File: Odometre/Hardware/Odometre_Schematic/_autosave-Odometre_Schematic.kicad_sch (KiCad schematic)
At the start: 9 parts, among them IC1 STM32C092FCP6, J1 Conn_01x04_Pin, J2 Conn_01x08_Pin, U1 MCP2562-E-SN, U2 LM1117DT-3.3

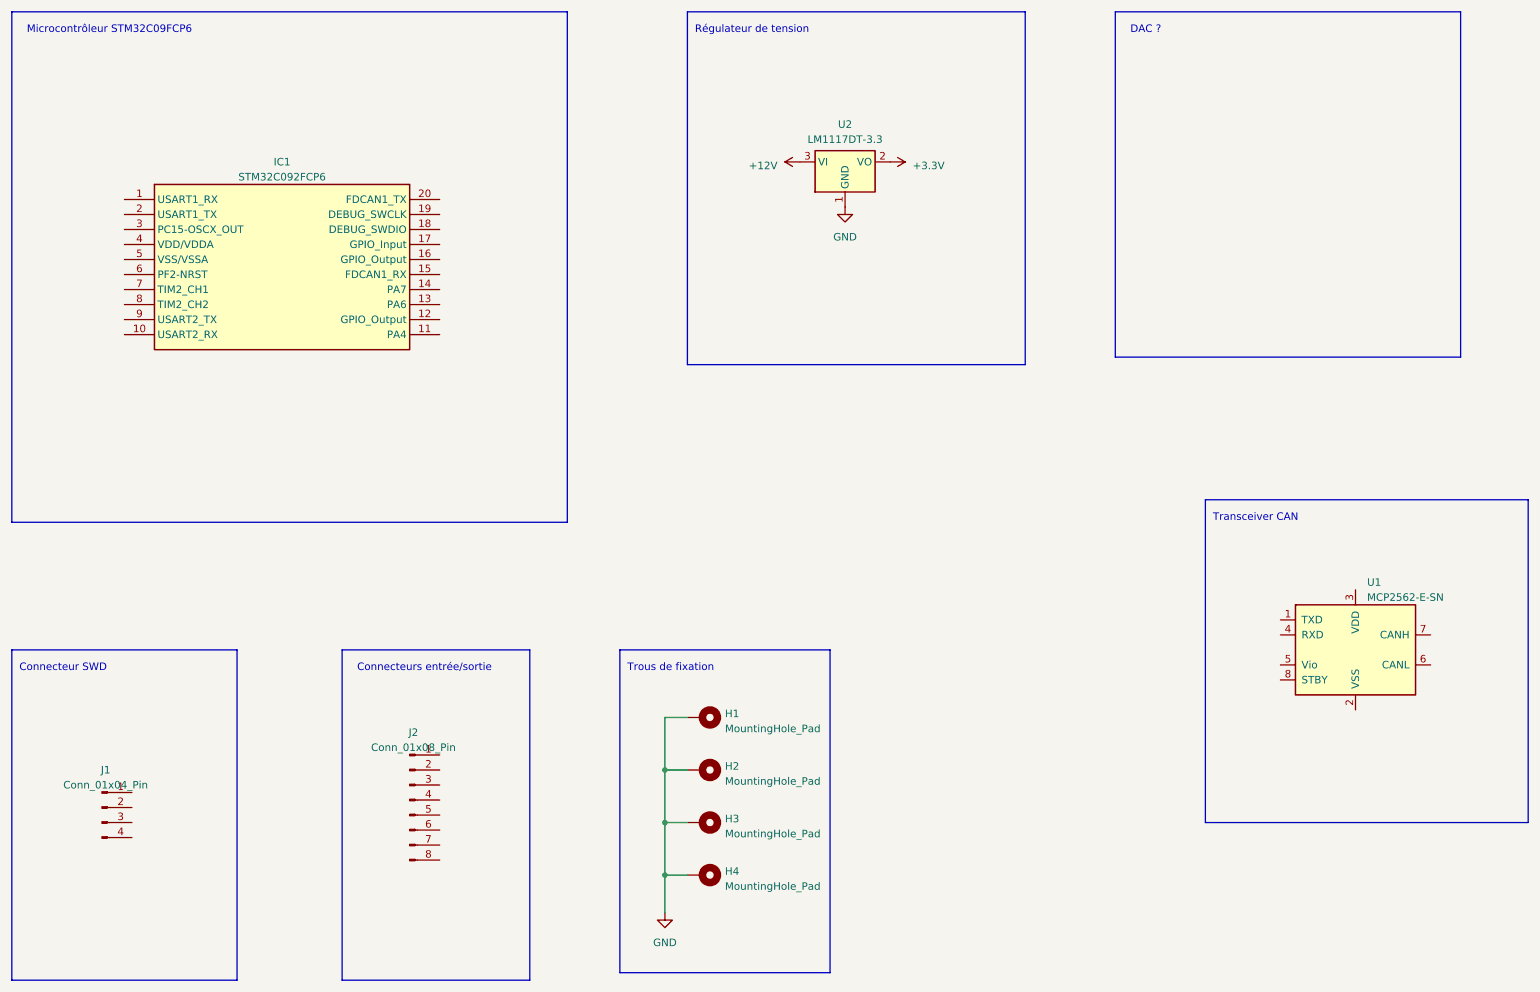
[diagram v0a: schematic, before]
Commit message: autosave kicad
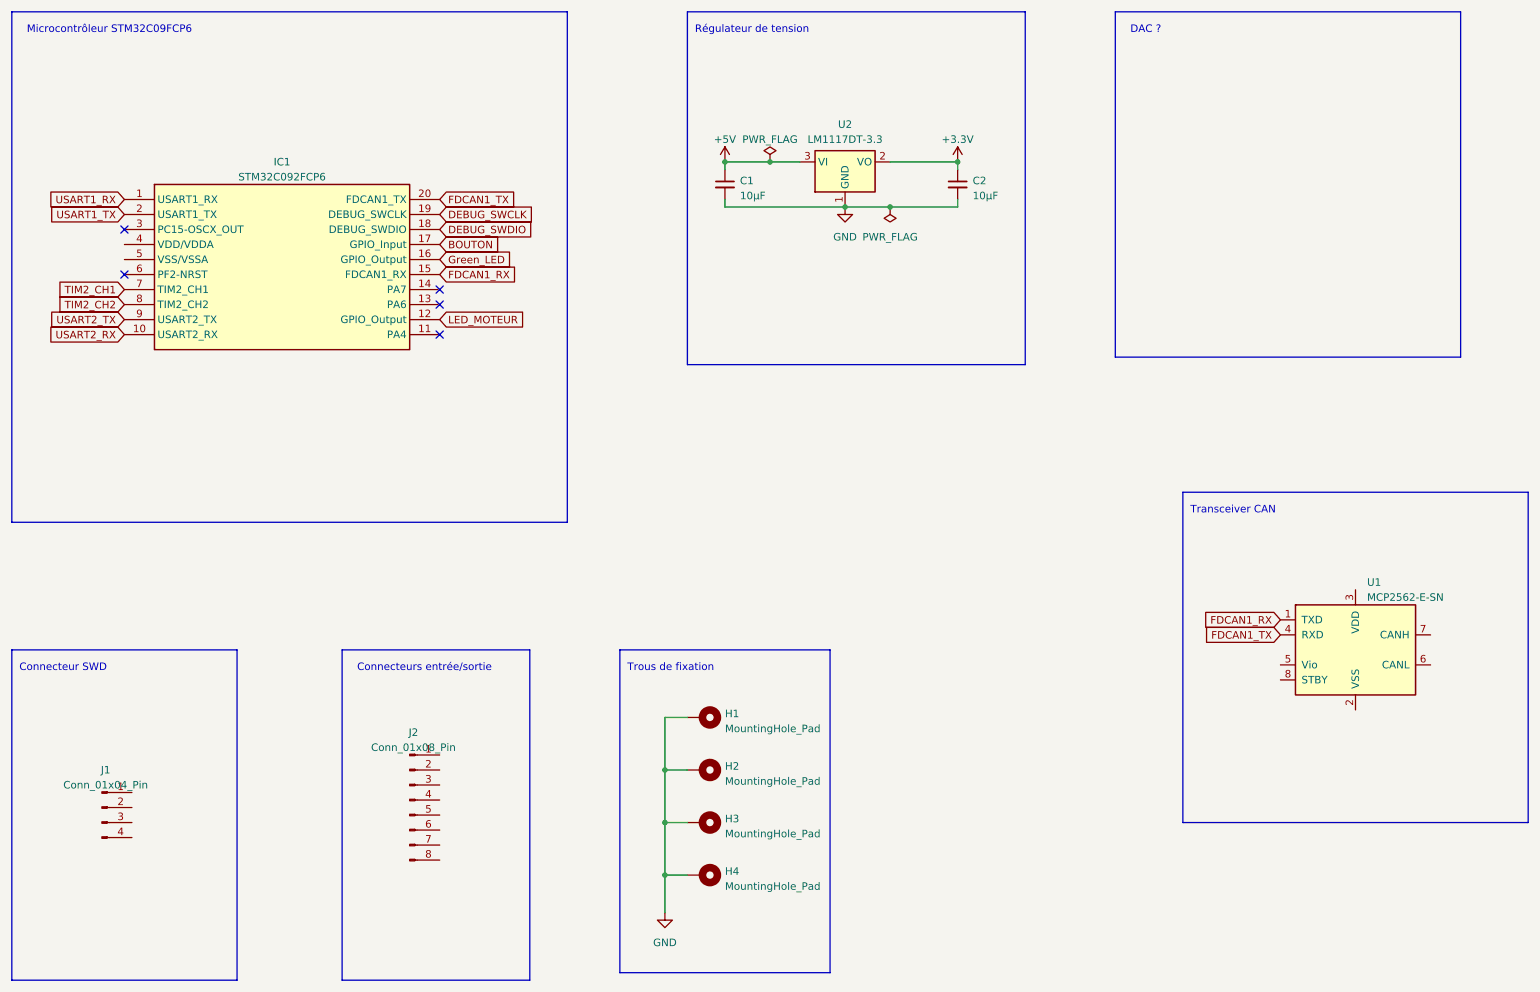
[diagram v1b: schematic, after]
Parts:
- added C1, C2: 10µF, symbol Device:C_Small
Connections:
- net +3.3V: now also C2.1
- net GND: now also C1.2, C2.2
- net FDCAN1_RX: now reaches U1.1 (TXD)
- net FDCAN1_RX: now also IC1.15 (FDCAN1_RX)
- net FDCAN1_TX: now reaches U1.4 (RXD)
- net FDCAN1_TX: now also IC1.20 (FDCAN1_TX)
- net USART1_RX: now reaches IC1.1 (USART1_RX)
- net USART2_RX: now reaches IC1.10 (USART2_RX)
- net LED_MOTEUR: now reaches IC1.12 (GPIO_Output)
- net Green_LED: now reaches IC1.16 (GPIO_Output)
- net BOUTON: now reaches IC1.17 (GPIO_Input)
- net DEBUG_SWDIO: now reaches IC1.18 (DEBUG_SWDIO)
- net DEBUG_SWCLK: now reaches IC1.19 (DEBUG_SWCLK)
- net USART1_TX: now reaches IC1.2 (USART1_TX)
- net TIM2_CH1: now reaches IC1.7 (TIM2_CH1)
- net TIM2_CH2: now reaches IC1.8 (TIM2_CH2)
- net USART2_TX: now reaches IC1.9 (USART2_TX)
- net +12V renamed +5V
- net +5V: now also C1.1
- no-connect marks 0 -> 5
